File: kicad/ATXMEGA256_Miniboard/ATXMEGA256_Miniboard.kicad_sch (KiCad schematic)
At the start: 15 parts, among them J1 Conn_01x08_Socket, J2 Conn_01x08_Socket, J3 Conn_01x08_Socket, J4 Conn_01x08_Socket, J5 Conn_01x08_Socket, J6 Conn_01x08_Socket, SW1 SW_Push_Dual, U1 ATXMEGA256A3B-AU

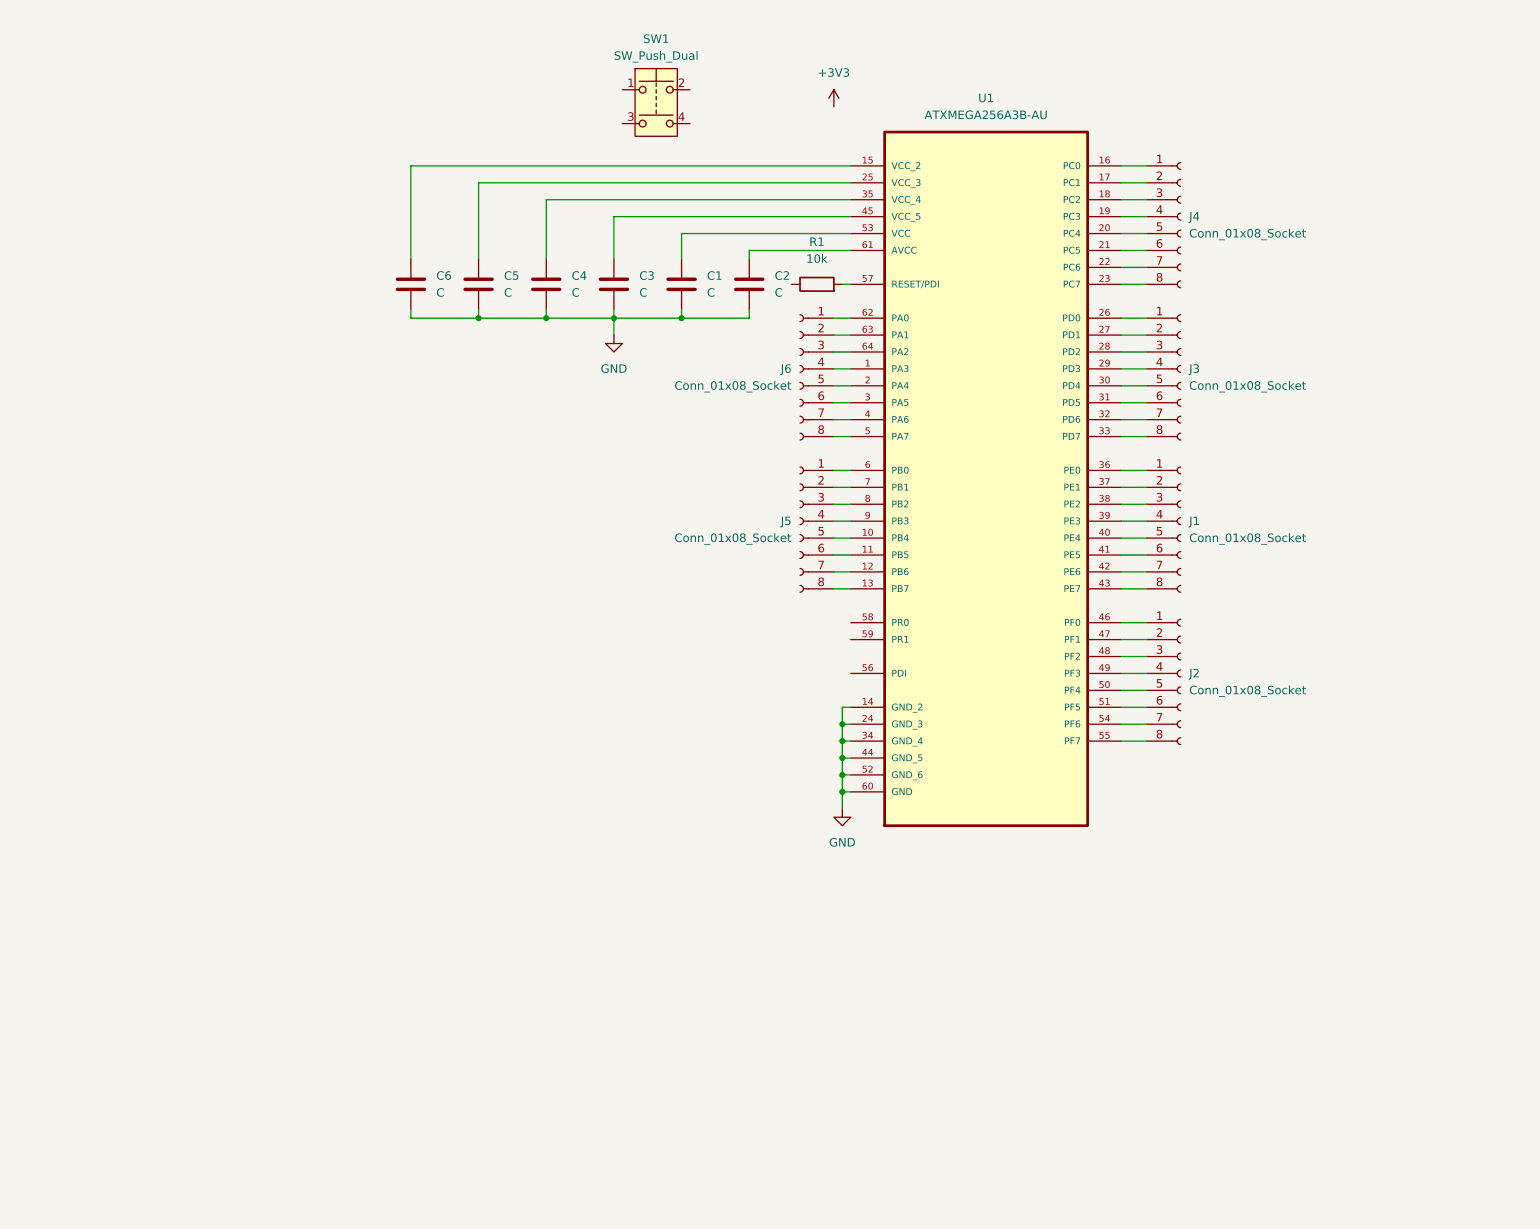
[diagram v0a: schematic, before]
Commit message: magistrale
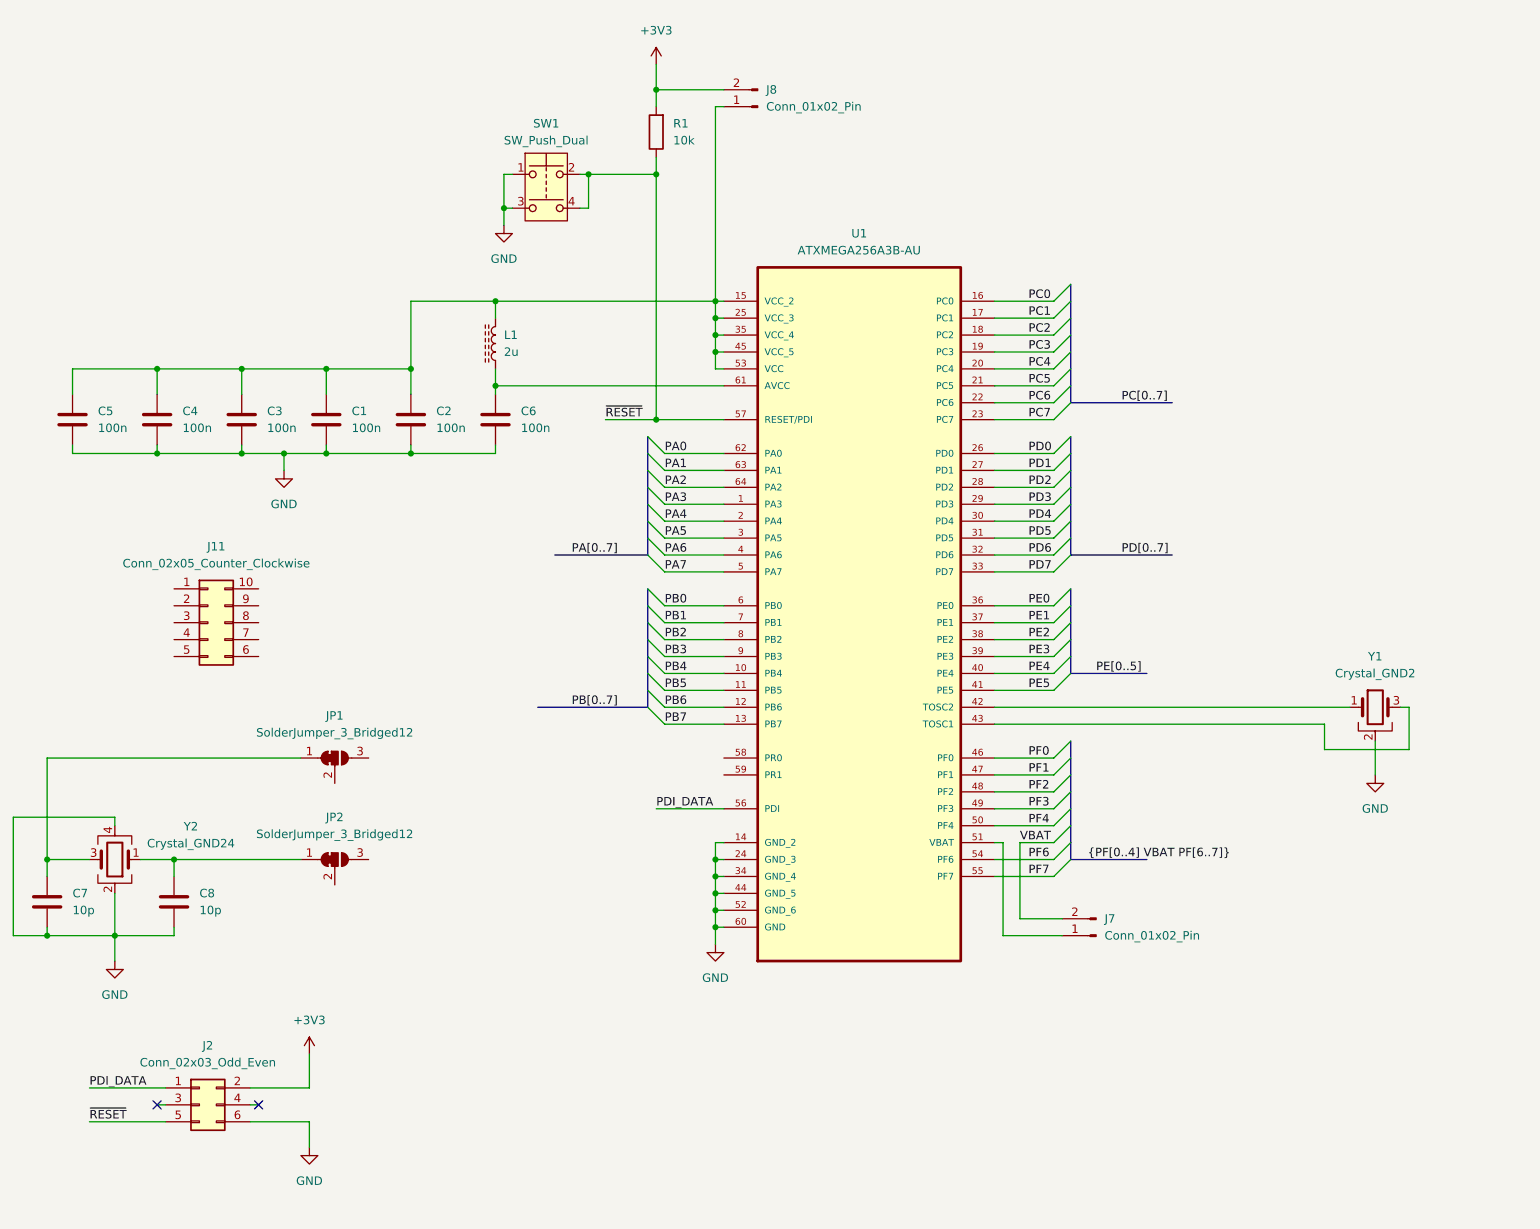
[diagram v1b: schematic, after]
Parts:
- removed J1, J2, J3, J4, J5, J6: Conn_01x08_Socket, symbol Connector:Conn_01x08_Socket
- added C7, C8: 10p, symbol Device:C
- added J11: Conn_02x05_Counter_Clockwise, symbol Connector_Generic:Conn_02x05_Counter_Clockwise
- added J2: Conn_02x03_Odd_Even, symbol Connector_Generic:Conn_02x03_Odd_Even
- added J7, J8: Conn_01x02_Pin, symbol Connector:Conn_01x02_Pin
- added JP1, JP2: SolderJumper_3_Bridged12, symbol Jumper:SolderJumper_3_Bridged12
- added L1: 2u, symbol Device:L_Ferrite
- added Y1: Crystal_GND2, symbol Device:Crystal_GND2
- added Y2: Crystal_GND24, symbol Device:Crystal_GND24
- C1, C2, C3, C4, C5, C6: value C -> 100n
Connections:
- net +3V3: now also R1.2, J2.2 (Pin_2), J8.2 (Pin_2)
- net GND: now also SW1.1, SW1.3, C7.1, C8.1, J2.6 (Pin_6), Y1.2, Y2.2, Y2.4
- net at C4.2, U1.35 (VCC_4): now also C1.2, C2.2, C3.2, C5.2, U1.15 (VCC_2), U1.25 (VCC_3), U1.45 (VCC_5), U1.53 (VCC), J8.1 (Pin_1), L1.2
- net ~{RESET}: now reaches R1.1
- net ~{RESET}: now also SW1.2, SW1.4, U1.57 (RESET/PDI), J2.5 (Pin_5)
- net PD0: now reaches U1.26 (PD0)
- net PD1: now reaches U1.27 (PD1)
- net PD2: now reaches U1.28 (PD2)
- net PD3: now reaches U1.29 (PD3)
- net PD4: now reaches U1.30 (PD4)
- net PD5: now reaches U1.31 (PD5)
- net PD6: now reaches U1.32 (PD6)
- net PD7: now reaches U1.33 (PD7)
- net PE0: now reaches U1.36 (PE0)
- net PE1: now reaches U1.37 (PE1)
- net PE2: now reaches U1.38 (PE2)
- net PE3: now reaches U1.39 (PE3)
- net PE4: now reaches U1.40 (PE4)
- net PE5: now reaches U1.41 (PE5)
- net at U1.42 (TOSC2): now also Y1.1
- net at U1.43 (TOSC1): now also Y1.3
- net PC0: now reaches U1.16 (PC0)
- net PC1: now reaches U1.17 (PC1)
- net PC2: now reaches U1.18 (PC2)
- net PC3: now reaches U1.19 (PC3)
- net PC4: now reaches U1.20 (PC4)
- net PC5: now reaches U1.21 (PC5)
- net PC6: now reaches U1.22 (PC6)
- net PC7: now reaches U1.23 (PC7)
- net PB0: now reaches U1.6 (PB0)
- net PB1: now reaches U1.7 (PB1)
- net PB2: now reaches U1.8 (PB2)
- net PB3: now reaches U1.9 (PB3)
- net PB4: now reaches U1.10 (PB4)
- net PB5: now reaches U1.11 (PB5)
- net PB6: now reaches U1.12 (PB6)
- net PB7: now reaches U1.13 (PB7)
- net at U1.61 (AVCC): now also C6.2, L1.1; no longer C2.2
- net PF0: now reaches U1.46 (PF0)
- net PF1: now reaches U1.47 (PF1)
- net PF2: now reaches U1.48 (PF2)
- net PF3: now reaches U1.49 (PF3)
- net PF4: now reaches U1.50 (PF4)
- net at U1.51 (VBAT): now also J7.1 (Pin_1)
- net PF6: now reaches U1.54 (PF6)
- net PF7: now reaches U1.55 (PF7)
- net PA3: now reaches U1.1 (PA3)
- net PA4: now reaches U1.2 (PA4)
- net PA5: now reaches U1.3 (PA5)
- net PA6: now reaches U1.4 (PA6)
- net PA7: now reaches U1.5 (PA7)
- net PDI_DATA: now reaches U1.56 (PDI)
- net PDI_DATA: now also J2.1 (Pin_1)
- net PA0: now reaches U1.62 (PA0)
- net PA1: now reaches U1.63 (PA1)
- net PA2: now reaches U1.64 (PA2)
- new net: C7.2, JP1.1 (A), Y2.3
- new net: C8.2, JP2.1 (A), Y2.1
- new net VBAT: J7.2 (Pin_2)
- no-connect marks 0 -> 2
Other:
- moved on the sheet: C1, C2, C3, C4, C5, R1, SW1, U1

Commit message: pierwsza wersja bez nazw i footprintów
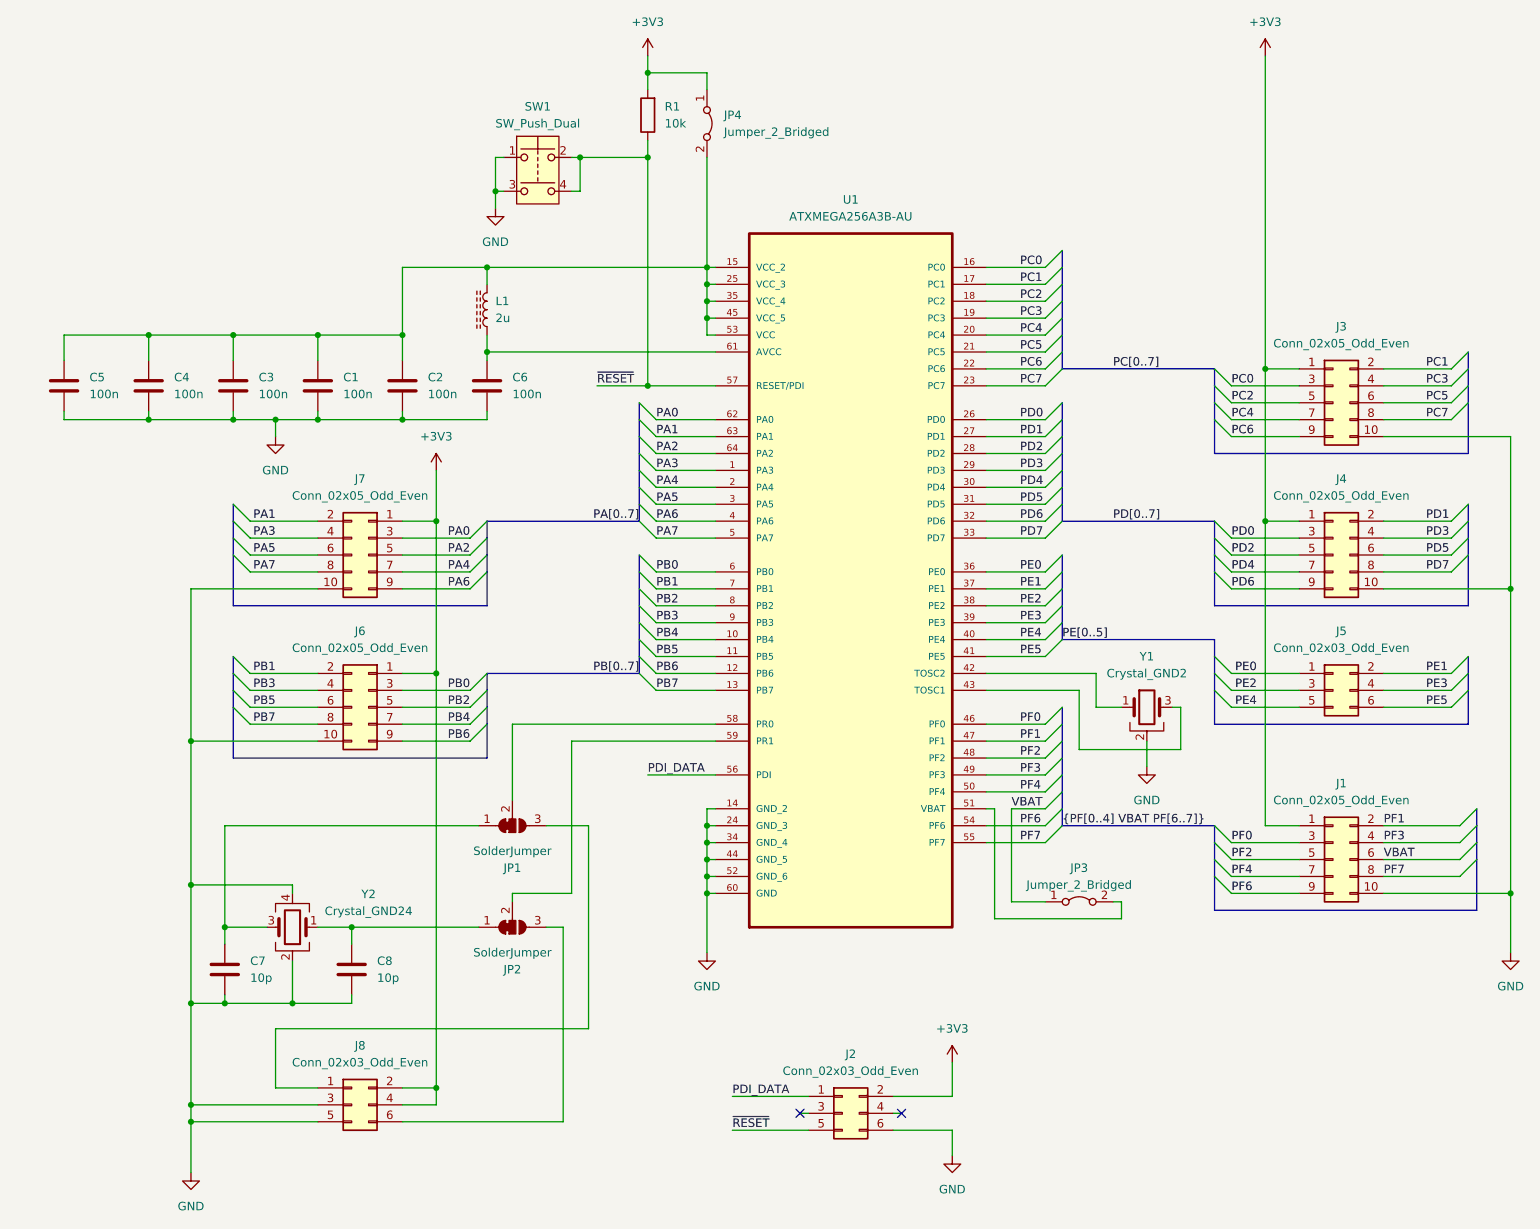
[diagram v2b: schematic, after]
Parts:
- removed J11: Conn_02x05_Counter_Clockwise, symbol Connector_Generic:Conn_02x05_Counter_Clockwise
- removed J7, J8: Conn_01x02_Pin, symbol Connector:Conn_01x02_Pin
- added J1, J3, J4, J6, J7: Conn_02x05_Odd_Even, symbol Connector_Generic:Conn_02x05_Odd_Even
- added J5, J8: Conn_02x03_Odd_Even, symbol Connector_Generic:Conn_02x03_Odd_Even
- added JP3, JP4: Jumper_2_Bridged, symbol Jumper:Jumper_2_Bridged
- JP1, JP2: value SolderJumper_3_Bridged12 -> SolderJumper
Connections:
- net +3V3: now also J1.1 (Pin_1), J3.1 (Pin_1), J4.1 (Pin_1), J6.1 (Pin_1), J7.1 (Pin_1), J8.2 (Pin_2), J8.4 (Pin_4), JP4.1 (A)
- net GND: now also J1.10 (Pin_10), J3.10 (Pin_10), J4.10 (Pin_10), J6.10 (Pin_10), J7.10 (Pin_10), J8.3 (Pin_3), J8.5 (Pin_5)
- net PA0: now also J7.3 (Pin_3)
- net PA1: now also J7.2 (Pin_2)
- net PA2: now also J7.5 (Pin_5)
- net PA3: now also J7.4 (Pin_4)
- net PA4: now also J7.7 (Pin_7)
- net PA5: now also J7.6 (Pin_6)
- net PA6: now also J7.9 (Pin_9)
- net PA7: now also J7.8 (Pin_8)
- net PB0: now also J6.3 (Pin_3)
- net PB1: now also J6.2 (Pin_2)
- net PB2: now also J6.5 (Pin_5)
- net PB3: now also J6.4 (Pin_4)
- net PB4: now also J6.7 (Pin_7)
- net PB5: now also J6.6 (Pin_6)
- net PB6: now also J6.9 (Pin_9)
- net PB7: now also J6.8 (Pin_8)
- net PC0: now also J3.3 (Pin_3)
- net PC1: now also J3.2 (Pin_2)
- net PC2: now also J3.5 (Pin_5)
- net PC3: now also J3.4 (Pin_4)
- net PC4: now also J3.7 (Pin_7)
- net PC5: now also J3.6 (Pin_6)
- net PC6: now also J3.9 (Pin_9)
- net PC7: now also J3.8 (Pin_8)
- net PD0: now also J4.3 (Pin_3)
- net PD1: now also J4.2 (Pin_2)
- net PD2: now also J4.5 (Pin_5)
- net PD3: now also J4.4 (Pin_4)
- net PD4: now also J4.7 (Pin_7)
- net PD5: now also J4.6 (Pin_6)
- net PD6: now also J4.9 (Pin_9)
- net PD7: now also J4.8 (Pin_8)
- net PE0: now also J5.1 (Pin_1)
- net PE1: now also J5.2 (Pin_2)
- net PE2: now also J5.3 (Pin_3)
- net PE3: now also J5.4 (Pin_4)
- net PE4: now also J5.5 (Pin_5)
- net PE5: now also J5.6 (Pin_6)
- net PF0: now also J1.3 (Pin_3)
- net PF1: now also J1.2 (Pin_2)
- net PF2: now also J1.5 (Pin_5)
- net PF3: now also J1.4 (Pin_4)
- net PF4: now also J1.7 (Pin_7)
- net PF6: now also J1.9 (Pin_9)
- net PF7: now also J1.8 (Pin_8)
- net VBAT: now also J1.6 (Pin_6), JP3.1 (A)
- net at C1.2, C2.2, C3.2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: now also JP4.2 (B)
- net at JP1.2 (C): now also U1.58 (PR0)
- net at JP1.3 (B): now also J8.1 (Pin_1)
- net at U1.51 (VBAT): now also JP3.2 (B)
- net at JP2.2 (C): now also U1.59 (PR1)
- net at JP2.3 (B): now also J8.6 (Pin_6)
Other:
- moved on the sheet: C1, C2, C3, C4, C5, C6, C7, C8, J2, JP1, JP2, L1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
